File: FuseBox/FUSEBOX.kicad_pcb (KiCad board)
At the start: 6 copper layers, 411.7 x 161.7 mm, 172 parts, among them J1 UJ31CHG2SMTTR, J10 901301150, J11 901301150, J12 901301240, J2 702462004, J3 702462004, J4 702462004, J5 702462004, J6 901301150, J7 702462004, J8 61301611121, J9 901301150, U1 TPS61040DBVR, U10 EC11E183440C, U11 EC11E183440C, U12 EC11E183440C, U13 EC11E183440C, U14 EC11E183440C, U2 LT3030EFETRPBF, U3 STM32F407VGTx, U4 ICE40HX8KCT256, U5 EC11E183440C, U6 EC11E183440C, U7 EC11E183440C, U8 EC11E183440C, U9 EC11E183440C, X1 STDCSU18M

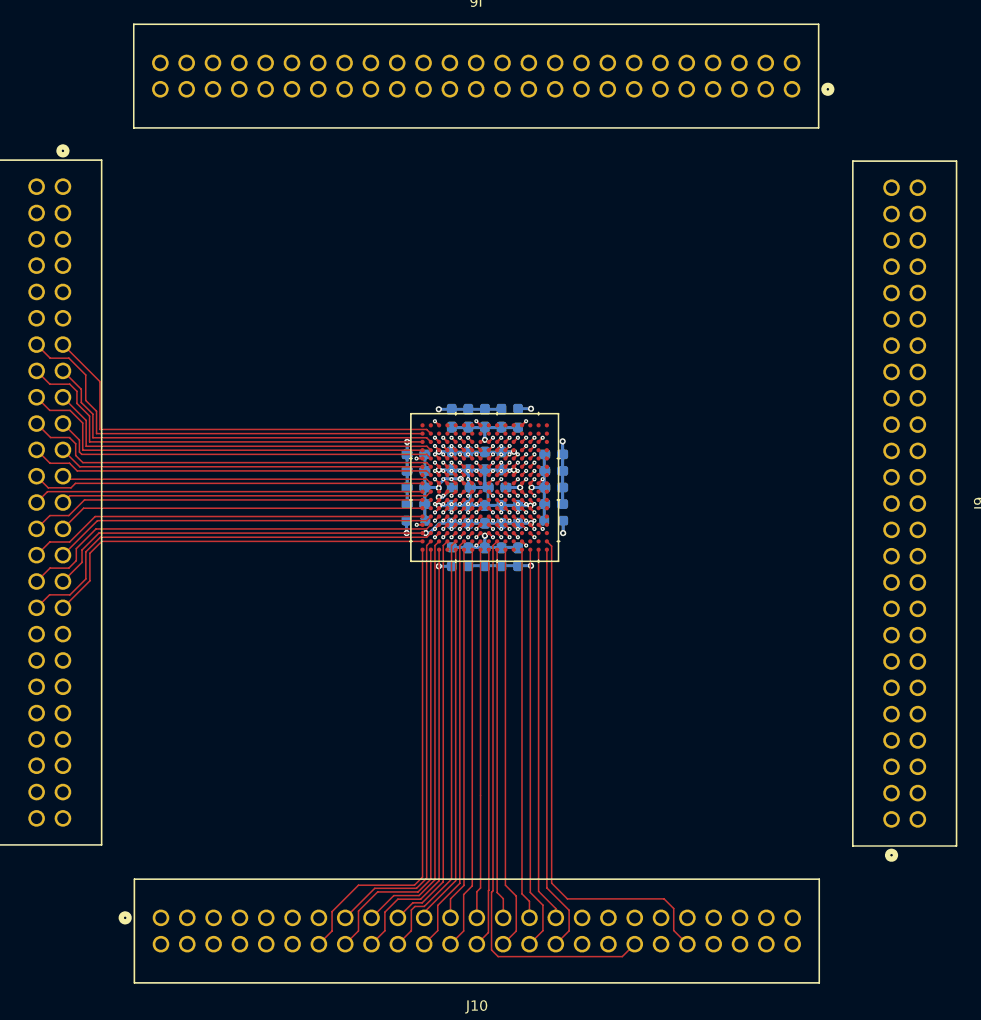
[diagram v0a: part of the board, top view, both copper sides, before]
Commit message: more traces
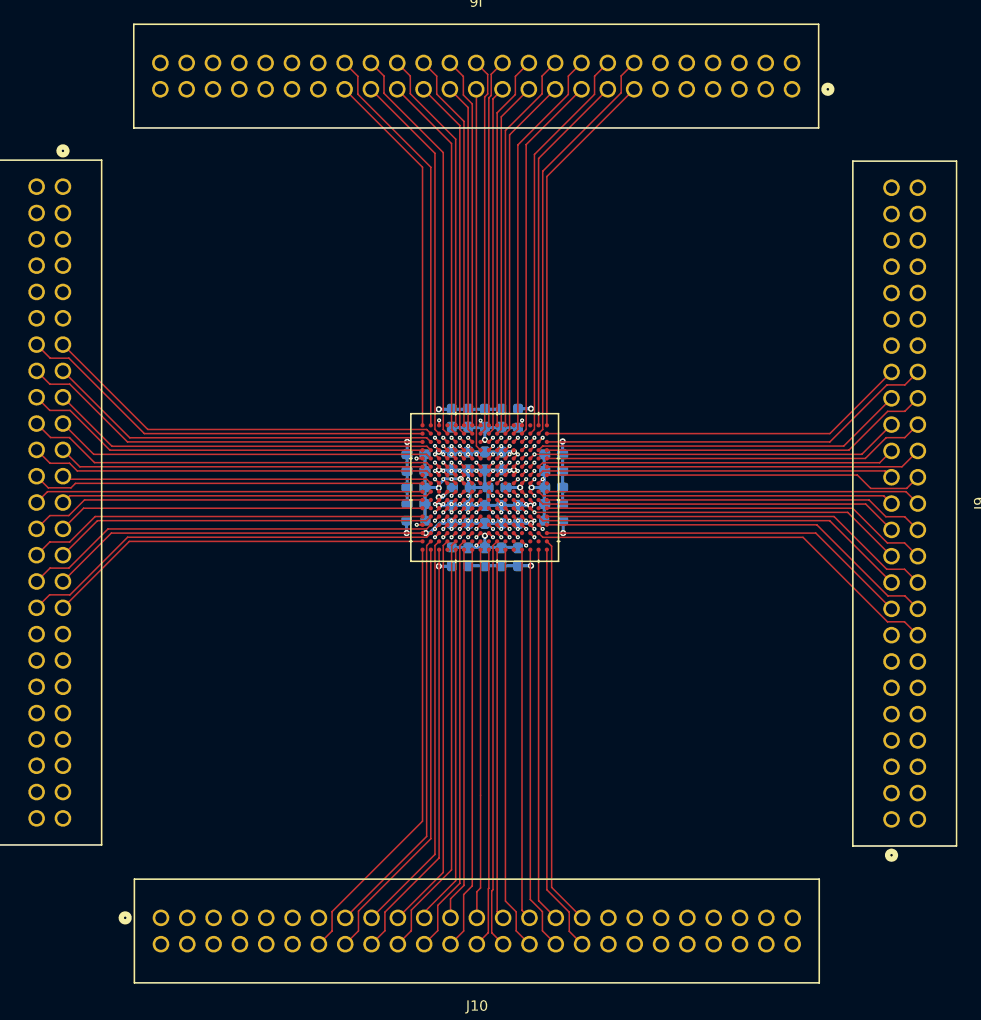
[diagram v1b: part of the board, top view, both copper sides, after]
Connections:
- J10 pad 2: /ICE40HX/ICE_B2_80 -> /ICE40HX/ICE_B2_68
- J10 pad 28: /ICE40HX/ICE_B2_89 -> /ICE40HX/ICE_B2_84
- J10 pad 3: /ICE40HX/ICE_B2_68 -> /ICE40HX/ICE_B2_80
- J10 pad 30: /ICE40HX/ICE_B2_92 -> /ICE40HX/ICE_B2_89
- J10 pad 32: /ICE40HX/ICE_B2_100 -> /ICE40HX/ICE_B2_92
- J10 pad 33: /ICE40HX/ICE_B2_83 -> /ICE40HX/ICE_B2_102
- J10 pad 34: /ICE40HX/ICE_B2_78 -> /ICE40HX/ICE_B2_100
- J10 pad 35: /ICE40HX/ICE_B2_86 -> /ICE40HX/ICE_B2_78
- J10 pad 36: /ICE40HX/ICE_B2_87 -> /ICE40HX/ICE_B2_83
- J10 pad 37: /ICE40HX/ICE_B2_93 -> /ICE40HX/ICE_B2_87
- J10 pad 38: /ICE40HX/ICE_B2_84 -> /ICE40HX/ICE_B2_86
- J10 pad 39: /ICE40HX/ICE_B2_98 -> /ICE40HX/ICE_B2_99
- J10 pad 4: /ICE40HX/ICE_B2_85 -> /ICE40HX/ICE_B2_74
- J10 pad 40: /ICE40HX/ICE_B2_99 -> /ICE40HX/ICE_B2_93
- J10 pad 42: /ICE40HX/ICE_B2_102 -> /ICE40HX/ICE_B2_98
- J10 pad 5: /ICE40HX/ICE_B2_74 -> /ICE40HX/ICE_B2_85
- J6 pad 13: unconnected-(J6-Pad13) -> /ICE40HX/ICE_T_176
- J6 pad 14: unconnected-(J6-Pad14) -> /ICE40HX/ICE_T_169
- J6 pad 15: unconnected-(J6-Pad15) -> /ICE40HX/ICE_T_177
- J6 pad 16: unconnected-(J6-Pad16) -> /ICE40HX/ICE_T_171
- J6 pad 17: unconnected-(J6-Pad17) -> /ICE40HX/ICE_T_178
- J6 pad 18: unconnected-(J6-Pad18) -> /ICE40HX/ICE_T_182
- J6 pad 19: unconnected-(J6-Pad19) -> /ICE40HX/ICE_T_184
- J6 pad 20: unconnected-(J6-Pad20) -> /ICE40HX/ICE_T_187
- J6 pad 21: unconnected-(J6-Pad21) -> /ICE40HX/ICE_T_183
- J6 pad 22: unconnected-(J6-Pad22) -> /ICE40HX/ICE_T_186
- J6 pad 23: unconnected-(J6-Pad23) -> /ICE40HX/ICE_T_199
- J6 pad 24: unconnected-(J6-Pad24) -> /ICE40HX/ICE_T_194
- J6 pad 25: unconnected-(J6-Pad25) -> /ICE40HX/ICE_T_200
- J6 pad 26: unconnected-(J6-Pad26) -> /ICE40HX/ICE_T_203
- J6 pad 27: unconnected-(J6-Pad27) -> /ICE40HX/ICE_T_207
- J6 pad 28: unconnected-(J6-Pad28) -> /ICE40HX/ICE_T_205
- J6 pad 29: unconnected-(J6-Pad29) -> /ICE40HX/ICE_T_208
- J6 pad 30: unconnected-(J6-Pad30) -> /ICE40HX/ICE_T_211
- J6 pad 31: unconnected-(J6-Pad31) -> /ICE40HX/ICE_T_214
- J6 pad 32: unconnected-(J6-Pad32) -> /ICE40HX/ICE_T_213
- J6 pad 33: unconnected-(J6-Pad33) -> /ICE40HX/ICE_T_223
- J6 pad 34: unconnected-(J6-Pad34) -> /ICE40HX/ICE_T_216
- J6 pad 35: unconnected-(J6-Pad35) -> /ICE40HX/ICE_T_220
- J6 pad 36: unconnected-(J6-Pad36) -> /ICE40HX/ICE_T_218
- J9 pad 16: unconnected-(J9-Pad16) -> /ICE40HX/ICE_R_112
- J9 pad 17: unconnected-(J9-Pad17) -> /ICE40HX/ICE_R_113
- J9 pad 18: unconnected-(J9-Pad18) -> /ICE40HX/ICE_R_117
- J9 pad 19: unconnected-(J9-Pad19) -> /ICE40HX/ICE_R_123
- J9 pad 20: unconnected-(J9-Pad20) -> /ICE40HX/ICE_R_121
- J9 pad 21: unconnected-(J9-Pad21) -> /ICE40HX/ICE_R_119
- J9 pad 22: unconnected-(J9-Pad22) -> /ICE40HX/ICE_R_127
- J9 pad 23: unconnected-(J9-Pad23) -> /ICE40HX/ICE_R_131
- J9 pad 24: unconnected-(J9-Pad24) -> /ICE40HX/ICE_R_133
- J9 pad 25: unconnected-(J9-Pad25) -> /ICE40HX/ICE_R_130
- J9 pad 26: unconnected-(J9-Pad26) -> /ICE40HX/ICE_R_138
- J9 pad 27: unconnected-(J9-Pad27) -> /ICE40HX/ICE_R_145
- J9 pad 28: unconnected-(J9-Pad28) -> /ICE40HX/ICE_R_143
- J9 pad 29: unconnected-(J9-Pad29) -> /ICE40HX/ICE_R_149
- J9 pad 30: unconnected-(J9-Pad30) -> /ICE40HX/ICE_R_147
- J9 pad 31: unconnected-(J9-Pad31) -> /ICE40HX/ICE_R_160
- J9 pad 32: unconnected-(J9-Pad32) -> /ICE40HX/ICE_R_151
- J9 pad 33: unconnected-(J9-Pad33) -> /ICE40HX/ICE_R_157
- J9 pad 34: unconnected-(J9-Pad34) -> /ICE40HX/ICE_R_153
- J9 pad 35: unconnected-(J9-Pad35) -> /ICE40HX/ICE_R_165
- J9 pad 36: unconnected-(J9-Pad36) -> /ICE40HX/ICE_R_161
- U4 pad A1: unconnected-(U4B-IOT_220-PadA1) -> /ICE40HX/ICE_T_220
- U4 pad A10: unconnected-(U4B-IOT_186-PadA10) -> /ICE40HX/ICE_T_186
- U4 pad A11: unconnected-(U4B-IOT_187-PadA11) -> /ICE40HX/ICE_T_187
- U4 pad A15: unconnected-(U4B-IOT_177-PadA15) -> /ICE40HX/ICE_T_177
- U4 pad A16: unconnected-(U4B-IOT_176-PadA16) -> /ICE40HX/ICE_T_176
- U4 pad A2: unconnected-(U4B-IOT_218-PadA2) -> /ICE40HX/ICE_T_218
- U4 pad A5: unconnected-(U4B-IOT_213-PadA5) -> /ICE40HX/ICE_T_213
- U4 pad A6: unconnected-(U4B-IOT_211-PadA6) -> /ICE40HX/ICE_T_211
- U4 pad A7: unconnected-(U4B-IOT_205-PadA7) -> /ICE40HX/ICE_T_205
- U4 pad A9: unconnected-(U4B-IOT_194-PadA9) -> /ICE40HX/ICE_T_194
- U4 pad B10: unconnected-(U4B-IOT_183-PadB10) -> /ICE40HX/ICE_T_183
- U4 pad B11: unconnected-(U4B-IOT_184-PadB11) -> /ICE40HX/ICE_T_184
- U4 pad B12: unconnected-(U4B-IOT_182-PadB12) -> /ICE40HX/ICE_T_182
- U4 pad B13: unconnected-(U4B-IOT_178-PadB13) -> /ICE40HX/ICE_T_178
- U4 pad B14: unconnected-(U4B-IOT_171-PadB14) -> /ICE40HX/ICE_T_171
- U4 pad B15: unconnected-(U4B-IOT_169-PadB15) -> /ICE40HX/ICE_T_169
- U4 pad B16: unconnected-(U4C-IOR_165-PadB16) -> /ICE40HX/ICE_R_165
- U4 pad B3: unconnected-(U4B-IOT_223-PadB3) -> /ICE40HX/ICE_T_223
- U4 pad B4: unconnected-(U4B-IOT_216-PadB4) -> /ICE40HX/ICE_T_216
- U4 pad B5: unconnected-(U4B-IOT_214-PadB5) -> /ICE40HX/ICE_T_214
- U4 pad B6: unconnected-(U4B-IOT_208-PadB6) -> /ICE40HX/ICE_T_208
- U4 pad B7: unconnected-(U4B-IOT_207-PadB7) -> /ICE40HX/ICE_T_207
- U4 pad B8: unconnected-(U4B-IOT_203-PadB8) -> /ICE40HX/ICE_T_203
- U4 pad B9: unconnected-(U4B-IOT_199-PadB9) -> /ICE40HX/ICE_T_199
- U4 pad C16: unconnected-(U4C-IOR_161-PadC16) -> /ICE40HX/ICE_R_161
- U4 pad D15: unconnected-(U4C-IOR_157-PadD15) -> /ICE40HX/ICE_R_157
- U4 pad D16: unconnected-(U4C-IOR_153-PadD16) -> /ICE40HX/ICE_R_153
- U4 pad D8: unconnected-(U4B-IOT_200-PadD8) -> /ICE40HX/ICE_T_200
- U4 pad E14: unconnected-(U4C-IOR_160-PadE14) -> /ICE40HX/ICE_R_160
- U4 pad E16: unconnected-(U4C-IOR_151-PadE16) -> /ICE40HX/ICE_R_151
- U4 pad F15: unconnected-(U4C-IOR_149-PadF15) -> /ICE40HX/ICE_R_149
- U4 pad F16: unconnected-(U4C-IOR_147-PadF16) -> /ICE40HX/ICE_R_147
- U4 pad G15: unconnected-(U4C-IOR_145-PadG15) -> /ICE40HX/ICE_R_145
- U4 pad G16: unconnected-(U4C-IOR_143-PadG16) -> /ICE40HX/ICE_R_143
- U4 pad J15: unconnected-(U4C-IOR_130-PadJ15) -> /ICE40HX/ICE_R_130
- U4 pad J16: unconnected-(U4C-IOR_138-PadJ16) -> /ICE40HX/ICE_R_138
- U4 pad K15: unconnected-(U4C-IOR_131-PadK15) -> /ICE40HX/ICE_R_131
- U4 pad K16: unconnected-(U4C-IOR_133-PadK16) -> /ICE40HX/ICE_R_133
- U4 pad L14: unconnected-(U4C-IOR_119-PadL14) -> /ICE40HX/ICE_R_119
- U4 pad L16: unconnected-(U4C-IOR_127-PadL16) -> /ICE40HX/ICE_R_127
- U4 pad M15: unconnected-(U4C-IOR_123-PadM15) -> /ICE40HX/ICE_R_123
- U4 pad M16: unconnected-(U4C-IOR_121-PadM16) -> /ICE40HX/ICE_R_121
- U4 pad N16: unconnected-(U4C-IOR_117-PadN16) -> /ICE40HX/ICE_R_117
- U4 pad P15: unconnected-(U4C-IOR_112-PadP15) -> /ICE40HX/ICE_R_112
- U4 pad P16: unconnected-(U4C-IOR_113-PadP16) -> /ICE40HX/ICE_R_113
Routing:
- net /ICE40HX/ICE_R_112: track 0.00 -> 40.7 mm
- net /ICE40HX/ICE_T_169: track 0.00 -> 39.6 mm
- net /ICE40HX/ICE_R_117: track 0.00 -> 39.2 mm
- net /ICE40HX/ICE_T_171: track 0.00 -> 38.9 mm
- net /ICE40HX/ICE_T_216: track 0.00 -> 38.8 mm
- net /ICE40HX/ICE_R_161: track 0.00 -> 38.6 mm
- net /ICE40HX/ICE_T_182: track 0.00 -> 38.5 mm
- net /ICE40HX/ICE_R_121: track 0.00 -> 38.4 mm
- net /ICE40HX/ICE_T_218: track 0.00 -> 38.4 mm
- net /ICE40HX/ICE_R_153: track 0.00 -> 37.9 mm
- net /ICE40HX/ICE_R_127: track 0.00 -> 37.7 mm
- net /ICE40HX/ICE_T_213: track 0.00 -> 37.3 mm
- net /ICE40HX/ICE_R_151: track 0.00 -> 37.2 mm
- net /ICE40HX/ICE_R_133: track 0.00 -> 37.0 mm
- net /ICE40HX/ICE_T_187: track 0.00 -> 37.0 mm
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
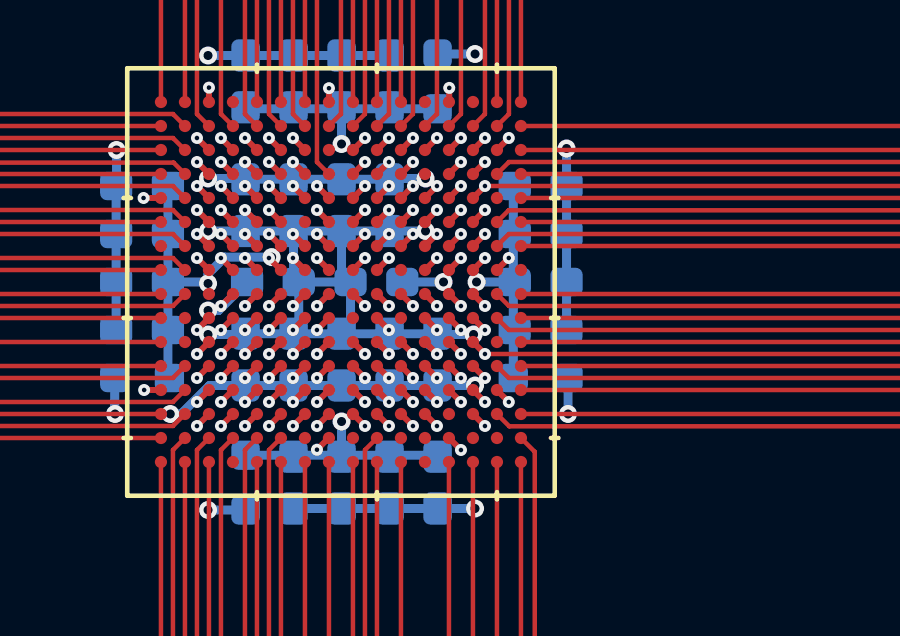
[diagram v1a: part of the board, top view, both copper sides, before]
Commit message: added again some traces
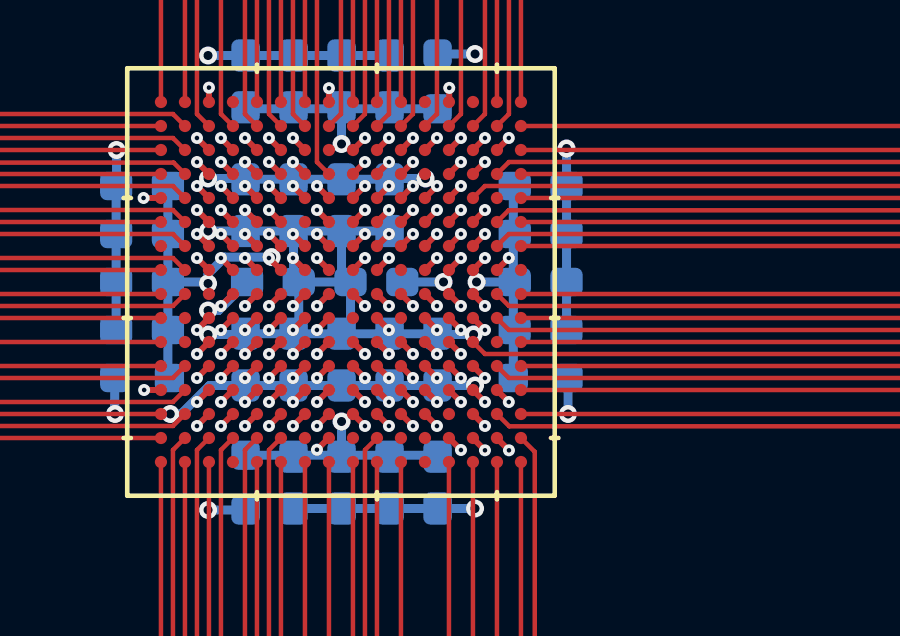
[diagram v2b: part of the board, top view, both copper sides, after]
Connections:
- J9 pad 1: unconnected-(J9-Pad1) -> /ICE40HX/ICE_R_136
- J9 pad 10: unconnected-(J9-Pad10) -> /ICE40HX/ICE_R_116
- J9 pad 11: unconnected-(J9-Pad11) -> /ICE40HX/ICE_R_118
- J9 pad 12: unconnected-(J9-Pad12) -> /ICE40HX/ICE_R_128
- J9 pad 13: unconnected-(J9-Pad13) -> /ICE40HX/ICE_R_129
- J9 pad 14: unconnected-(J9-Pad14) -> /ICE40HX/ICE_R_137
- J9 pad 15: unconnected-(J9-Pad15) -> /ICE40HX/ICE_R_134
- J9 pad 2: unconnected-(J9-Pad2) -> /ICE40HX/ICE_R_126
- J9 pad 3: unconnected-(J9-Pad3) -> /ICE40HX/ICE_R_122
- J9 pad 37: unconnected-(J9-Pad37) -> /ICE40HX/ICE_R_150
- J9 pad 38: unconnected-(J9-Pad38) -> /ICE40HX/ICE_R_142
- J9 pad 39: unconnected-(J9-Pad39) -> /ICE40HX/ICE_R_155
- J9 pad 4: unconnected-(J9-Pad4) -> /ICE40HX/ICE_R_120
- J9 pad 40: unconnected-(J9-Pad40) -> /ICE40HX/ICE_R_152
- J9 pad 41: unconnected-(J9-Pad41) -> /ICE40HX/ICE_R_166
- J9 pad 42: unconnected-(J9-Pad42) -> /ICE40HX/ICE_R_162
- J9 pad 43: unconnected-(J9-Pad43) -> /ICE40HX/ICE_R_154
- J9 pad 44: unconnected-(J9-Pad44) -> /ICE40HX/ICE_R_167
- J9 pad 45: unconnected-(J9-Pad45) -> /ICE40HX/ICE_R_146
- J9 pad 46: unconnected-(J9-Pad46) -> /ICE40HX/ICE_R_156
- J9 pad 48: unconnected-(J9-Pad48) -> /ICE40HX/ICE_R_158
- J9 pad 5: unconnected-(J9-Pad5) -> /ICE40HX/ICE_R_110
- J9 pad 6: unconnected-(J9-Pad6) -> /ICE40HX/ICE_R_109
- J9 pad 7: unconnected-(J9-Pad7) -> /ICE40HX/ICE_R_111
- J9 pad 8: unconnected-(J9-Pad8) -> /ICE40HX/ICE_R_114
- J9 pad 9: unconnected-(J9-Pad9) -> /ICE40HX/ICE_R_115
- U4 pad D14: unconnected-(U4C-IOR_167-PadD14) -> /ICE40HX/ICE_R_167
- U4 pad E13: unconnected-(U4C-IOR_166-PadE13) -> /ICE40HX/ICE_R_166
- U4 pad F11: unconnected-(U4C-IOR_158-PadF11) -> /ICE40HX/ICE_R_158
- U4 pad F12: unconnected-(U4C-IOR_156-PadF12) -> /ICE40HX/ICE_R_156
- U4 pad F13: unconnected-(U4C-IOR_162-PadF13) -> /ICE40HX/ICE_R_162
- U4 pad F14: unconnected-(U4C-IOR_155-PadF14) -> /ICE40HX/ICE_R_155
- U4 pad G10: unconnected-(U4C-IOR_146-PadG10) -> /ICE40HX/ICE_R_146
- U4 pad G12: unconnected-(U4C-IOR_154-PadG12) -> /ICE40HX/ICE_R_154
- U4 pad G13: unconnected-(U4C-IOR_152-PadG13) -> /ICE40HX/ICE_R_152
- U4 pad G14: unconnected-(U4C-IOR_150-PadG14) -> /ICE40HX/ICE_R_150
- U4 pad H14: unconnected-(U4C-IOR_142-PadH14) -> /ICE40HX/ICE_R_142
- U4 pad J10: unconnected-(U4C-IOR_122-PadJ10) -> /ICE40HX/ICE_R_122
- U4 pad J11: unconnected-(U4C-IOR_126-PadJ11) -> /ICE40HX/ICE_R_126
- U4 pad J12: unconnected-(U4C-IOR_136-PadJ12) -> /ICE40HX/ICE_R_136
- U4 pad J13: unconnected-(U4C-IOR_137-PadJ13) -> /ICE40HX/ICE_R_137
- U4 pad J14: unconnected-(U4C-IOR_134-PadJ14) -> /ICE40HX/ICE_R_134
- U4 pad K12: unconnected-(U4C-IOR_120-PadK12) -> /ICE40HX/ICE_R_120
- U4 pad K13: unconnected-(U4C-IOR_128-PadK13) -> /ICE40HX/ICE_R_128
- U4 pad K14: unconnected-(U4C-IOR_129-PadK14) -> /ICE40HX/ICE_R_129
- U4 pad L12: unconnected-(U4C-IOR_116-PadL12) -> /ICE40HX/ICE_R_116
- U4 pad L13: unconnected-(U4C-IOR_118-PadL13) -> /ICE40HX/ICE_R_118
- U4 pad M13: unconnected-(U4C-IOR_114-PadM13) -> /ICE40HX/ICE_R_114
- U4 pad M14: unconnected-(U4C-IOR_115-PadM14) -> /ICE40HX/ICE_R_115
- U4 pad P14: unconnected-(U4C-IOR_111-PadP14) -> /ICE40HX/ICE_R_111
- U4 pad R14: unconnected-(U4C-IOR_109-PadR14) -> /ICE40HX/ICE_R_109
- U4 pad R15: unconnected-(U4C-IOR_110-PadR15) -> /ICE40HX/ICE_R_110
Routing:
- net /ICE40HX/ICE_R_120: track 0.00 -> 50.7 mm, vias 0 -> 1
- net /ICE40HX/ICE_R_122: track 0.00 -> 50.1 mm, vias 0 -> 1
- net /ICE40HX/ICE_R_156: track 0.00 -> 48.1 mm, vias 0 -> 1
- net /ICE40HX/ICE_R_116: track 0.00 -> 47.2 mm, vias 0 -> 1
- net /ICE40HX/ICE_R_114: track 0.00 -> 47.2 mm, vias 0 -> 1
- net /ICE40HX/ICE_R_109: track 0.00 -> 46.7 mm, vias 0 -> 1
- net /ICE40HX/ICE_R_126: track 0.00 -> 46.5 mm, vias 0 -> 1
- net /ICE40HX/ICE_R_136: track 0.00 -> 46.0 mm, vias 0 -> 1
- net /ICE40HX/ICE_R_158: track 0.00 -> 45.9 mm, vias 0 -> 1
- net /ICE40HX/ICE_R_128: track 0.00 -> 45.7 mm, vias 0 -> 1
- net /ICE40HX/ICE_R_162: track 0.00 -> 45.1 mm, vias 0 -> 1
- net /ICE40HX/ICE_R_137: track 0.00 -> 45.0 mm, vias 0 -> 1
- net /ICE40HX/ICE_R_154: track 0.00 -> 44.8 mm, vias 0 -> 1
- net /ICE40HX/ICE_R_167: track 0.00 -> 44.7 mm, vias 0 -> 1
- net /ICE40HX/ICE_R_152: track 0.00 -> 44.4 mm, vias 0 -> 1
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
